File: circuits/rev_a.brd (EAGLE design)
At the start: 160 x 100 mm, 5 parts

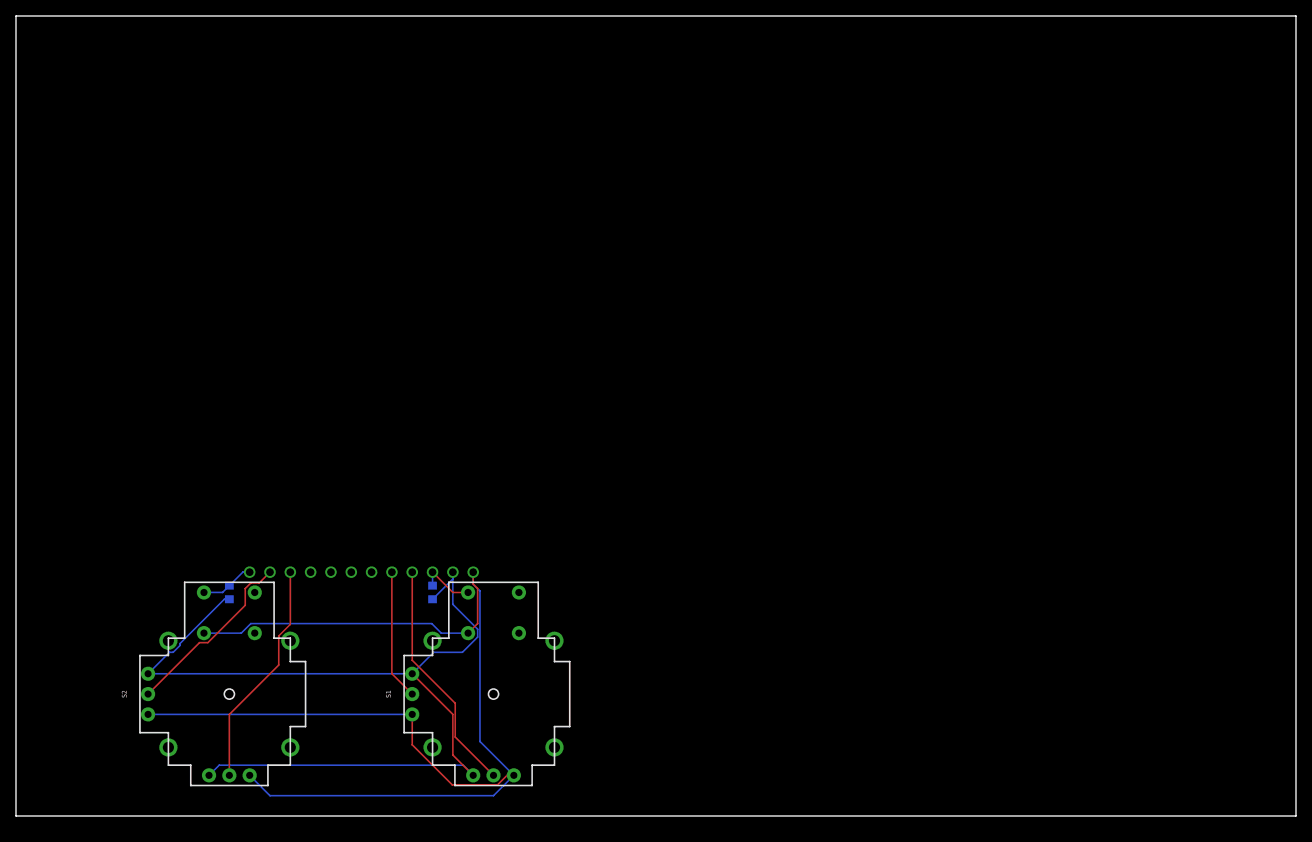
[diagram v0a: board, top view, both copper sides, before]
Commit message: Finished a rev a, but it's enormous.
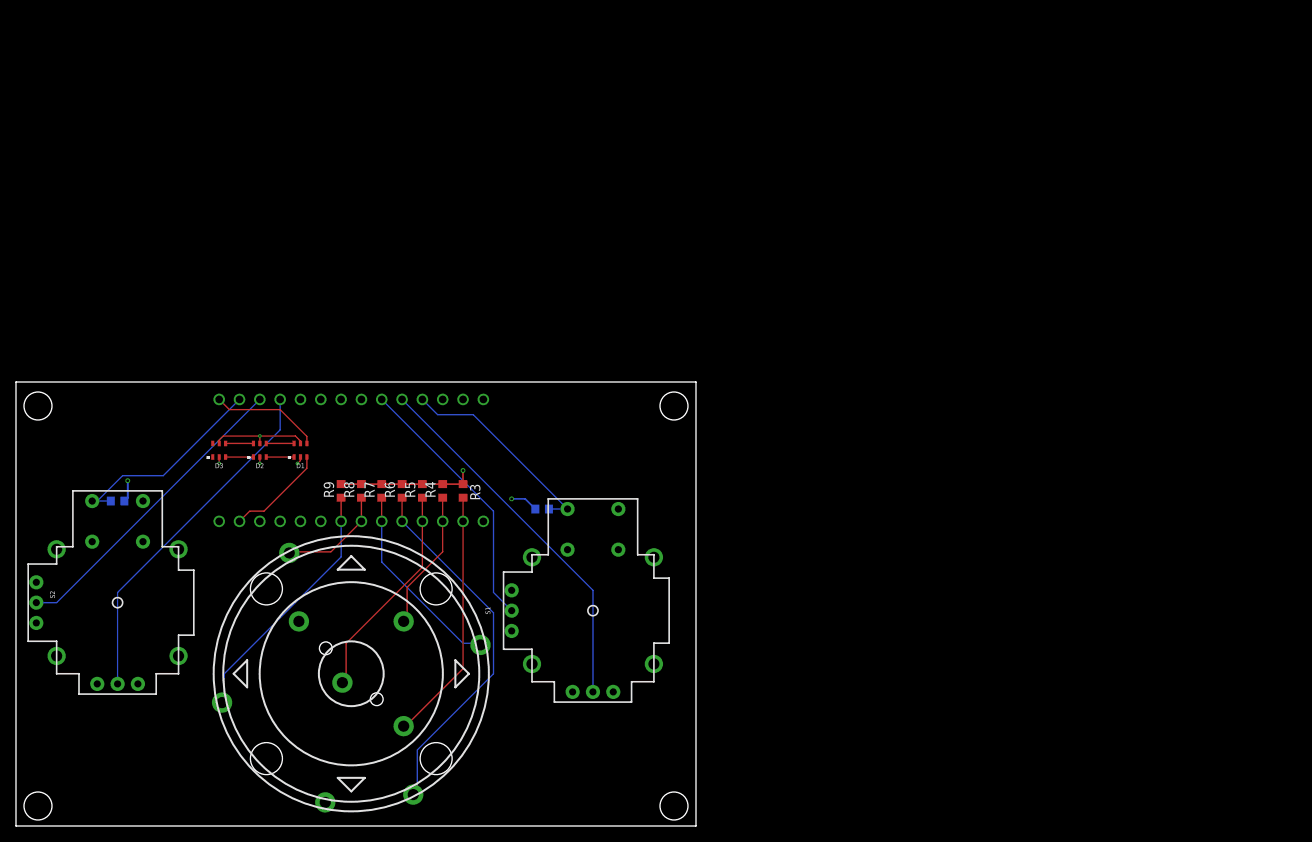
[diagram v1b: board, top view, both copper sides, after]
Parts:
- added D1, D2, D3: APA102-2020, SparkFun-LED:APA102-2020
- added R3: 10k, adafruit:R0603
- added R4, R5, R6, R7, R8, R9: (no value), adafruit:R0603
- added X1: ENCODER_ANO, custom:ENCODER_ANO
- MCU: value TEENSY_4.0-ANALOG-DEPIN -> TEENSY_4.0-NOBOTTOM; device Teensy-4.0:TEENSY_4.0-ANALOG-DEPIN -> Teensy-4.0:TEENSY_4.0-NOBOTTOM
- moved MCU 21.6 mm to (41.9, 44.5)
- moved S2 18.1 mm to (12.7, 26.7)
- moved R2 18.1 mm to (12.7, 39.4), turned to 0 degrees
- moved R1 17.2 mm to (65.8, 38.4), turned to 180 degrees
- moved S1 16.2 mm to (72.1, 25.7)
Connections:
- new net N$1: MCU.6, R9.1, X1.S5
- new net N$10: D2.SDO, D3.SDI
- new net N$11: D2.CKO, D3.CKI
- new net N$12: D1.CKI, MCU.13/SCK
- new net N$13: D1.SDI, MCU.11/MOSI
- new net N$2: MCU.5, R8.1, X1.S4
- new net N$3: MCU.4/CANRX, R7.1, X1.S3
- new net N$4: MCU.3/CANTX, R6.1, X1.S2
- new net N$5: MCU.2, R5.1, X1.S1
- new net N$6: MCU.1/TX, R4.1, X1.B
- new net N$7: MCU.0/RX, R3.2, X1.A
- new net N$8: D1.SDO, D2.SDI
- new net N$9: D1.CKO, D2.CKI
- net +3V3: now also D1.VDD, D2.VDD, D3.VDD, R3.1, R4.2, R5.2, R6.2, R7.2, R8.2, R9.2
- net GND: now also D1.GND, D2.GND, D3.GND, X1.COM_A, X1.COM_B
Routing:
- net GND: track 157.1 -> 2.57 mm, vias 0 -> 3
- net +3V3: track 121.0 -> 185.4 mm, vias 0 -> 4
- net N$4: track 0.00 -> 46.0 mm
- net N$1: track 0.00 -> 31.7 mm
- net N$7: track 0.00 -> 31.7 mm
- net N$5: track 0.00 -> 27.3 mm
- net N$3: track 0.00 -> 24.7 mm
- net S1: track 7.19 -> 26.1 mm
- net S2: track 6.77 -> 25.4 mm
- net N$6: track 0.00 -> 17.5 mm
- net HOR1: track 29.6 -> 46.4 mm
- net VERT1: track 16.3 -> 33.1 mm
- net VERT2: track 22.8 -> 38.5 mm
- net HOR2: track 28.6 -> 44.0 mm
- net N$12: track 0.00 -> 13.8 mm
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- added copper zone on layer 2, net GND
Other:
- board size 160 x 100 mm -> 85 x 55.5 mm
